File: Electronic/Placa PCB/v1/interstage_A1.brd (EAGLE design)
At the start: 82.5 x 29 mm, 11 parts, among them J1 0532611271, J3 0532611271, Q1 PMV16XNR, U1 LM70CIMM-3, U2 LM70CIMM-3

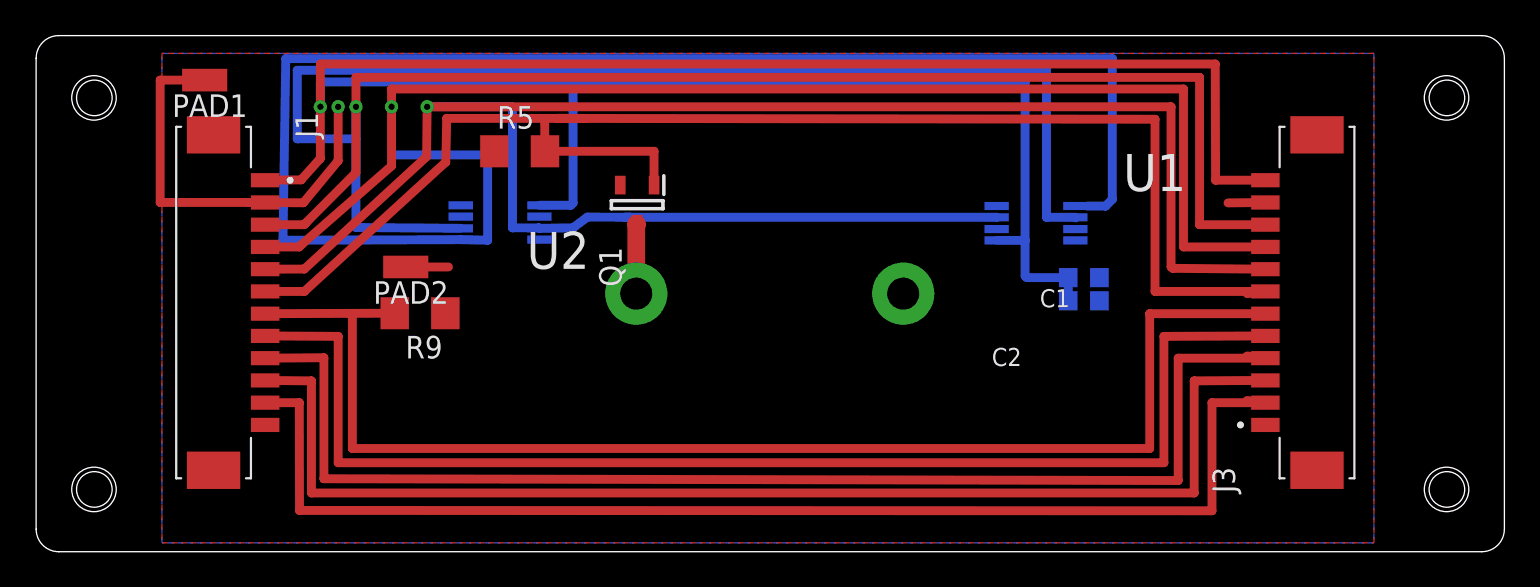
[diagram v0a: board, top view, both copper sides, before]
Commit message: Avance
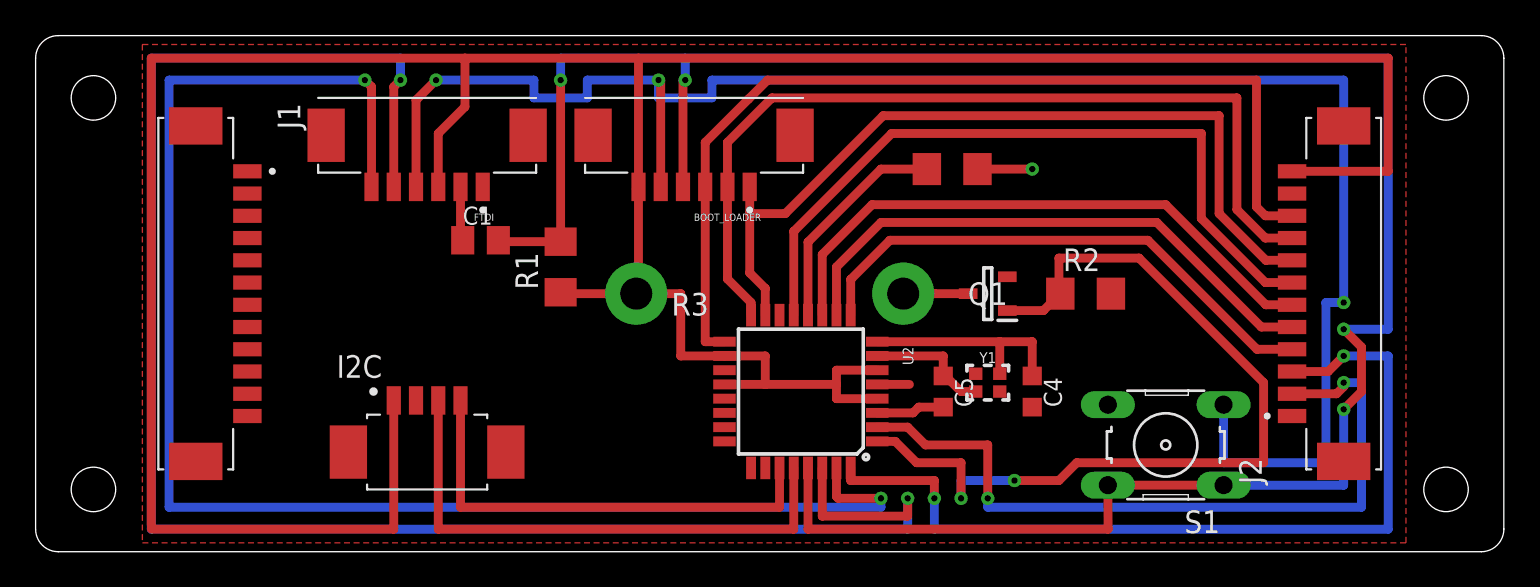
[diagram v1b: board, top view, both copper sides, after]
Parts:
- removed C2: 0.1pF, rcl:C0603K
- removed J3: 0532611271, picoblade:MOLEX_0532611271
- removed PAD1, PAD2: WIREPADSMD1,27-254, wirepad:SMD1,27-2,54
- removed R5, R9: 330 Ohm, rcl:R1206
- removed U1: LM70CIMM-3, LM70CIMM-3:SOP65P490X110-8N
- added BOOT_LOADER, FTDI: 0532610671, picoblade6:MOLEX_0532610671
- added C4, C5: 22pF, rcl:C0603K
- added I2C: 0532610471, 0532610471:MOLEX_0532610471
- added J2: 0532611271, picoblade:MOLEX_0532611271
- added R1: 10kohm, rcl:R1206
- added R2, R3: 330 Ohm, rcl:R1206
- added S1: (no value), switch-omron:B3F-10XX
- added Y1: 16MHz, SparkFun-Clocks:CRYSTAL-SMD-2.0X1.6MM
- C1: value 0.1pF -> 100nF; device rcl:C0603K -> rcl:C0805K
- U2: value LM70CIMM-3 -> ATMEGA328P_TQFP; device LM70CIMM-3:SOP65P490X110-8N -> SparkFun-IC-Microcontroller:TQFP32-08
- moved C1 34.0 mm to (25.0, 17.5), flipped to the top, turned to 0 degrees
- moved Q1 20.3 mm to (53.5, 14.5), turned to 180 degrees
- moved U2 19.4 mm to (43.0, 9.00), flipped to the top
- moved J1 1.12 mm to (9.00, 14.5)
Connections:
- net MOSFET renamed NICROMO
- removed net N$3: J3.1
- removed net N$4: R9.1
- new net DTR: C1.1, FTDI.2
- new net ICP: R3.1, U2.12
- new net INT1: Q1.1, R2.1, U2.1
- new net N$1: C5.1, U2.7, Y1.1
- new net N$2: C4.1, U2.8, Y1.3
- new net N$6: U2.14
- new net RST: BOOT_LOADER.4, C1.2, R1.2, S1.1, S1.2, U2.29
- new net RXD: FTDI.5, U2.30
- new net SCL: I2C.3, U2.28
- new net SDA: I2C.4, U2.27
- new net SWITCH: R3.2
- new net TXD: FTDI.6, U2.31
- net AIN0: now also J2.5, U2.10; no longer J1.8, J3.5
- net AIN1: now also J2.6, U2.11; no longer J1.7, J3.6, R9.2
- net GND: now also BOOT_LOADER.5, C4.2, C5.2, FTDI.4, I2C.2, J2.11, R2.2, S1.3, S1.4, U2.3, U2.5; no longer C1.2, C2.2, J1.2, J3.11, PAD1.1, PAD2.1, R5.1, U1.4, U2.4
- net INT0: now also J2.3, U2.32; no longer J1.10, J3.3
- net MISO: now also BOOT_LOADER.2, J2.9, U2.16; no longer J1.4, J3.9, U1.1, U2.1
- net MOSI: now also BOOT_LOADER.1, J2.8, U2.15; no longer J1.5, J3.8, U1.7, U2.7
- net OC1A: now also J2.7, U2.13; no longer J1.6, J3.7, Q1.1, R5.2
- net SCK: now also BOOT_LOADER.3, J2.10, U2.17; no longer J1.3, J3.10, U1.2, U2.2
- net T0: now also J2.2, U2.2; no longer J1.11, J3.2
- net T1: now also J2.4, U2.9; no longer J1.9, J3.4
- net VCC: now also BOOT_LOADER.6, FTDI.3, I2C.1, J2.12, R1.1, U2.18, U2.20, U2.4, U2.6; no longer C1.1, C2.1, J1.1, J3.12, U1.5, U2.5
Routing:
- net RST: track 0.00 -> 131.1 mm, vias 0 -> 4
- net MISO: track 161.6 -> 50.0 mm, vias 1 -> 0
- net RXD: track 0.00 -> 100.6 mm, vias 0 -> 2
- net SCK: track 142.9 -> 54.0 mm, vias 1 -> 0
- net TXD: track 0.00 -> 85.8 mm, vias 0 -> 2
- net GND: track 29.8 -> 104.7 mm, vias 1 -> 3
- net MOSI: track 109.8 -> 46.9 mm, vias 1 -> 0
- net INT1: track 0.00 -> 49.9 mm, vias 0 -> 2
- net VCC: track 134.6 -> 178.9 mm
- net OC1A: track 84.4 -> 41.3 mm
- net T1: track 70.9 -> 30.3 mm
- net AIN1: track 73.7 -> 33.3 mm
- net AIN0: track 70.4 -> 32.0 mm
- net SCL: track 0.00 -> 30.6 mm
- net T0: track 69.4 -> 42.4 mm, vias 0 -> 2
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- removed copper zone on layer 16, net GND
